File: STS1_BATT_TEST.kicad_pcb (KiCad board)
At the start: 2 copper layers, 81.8 x 46.9 mm, 6 parts, among them J1 TE 282834-6, J2 Conn_01x15

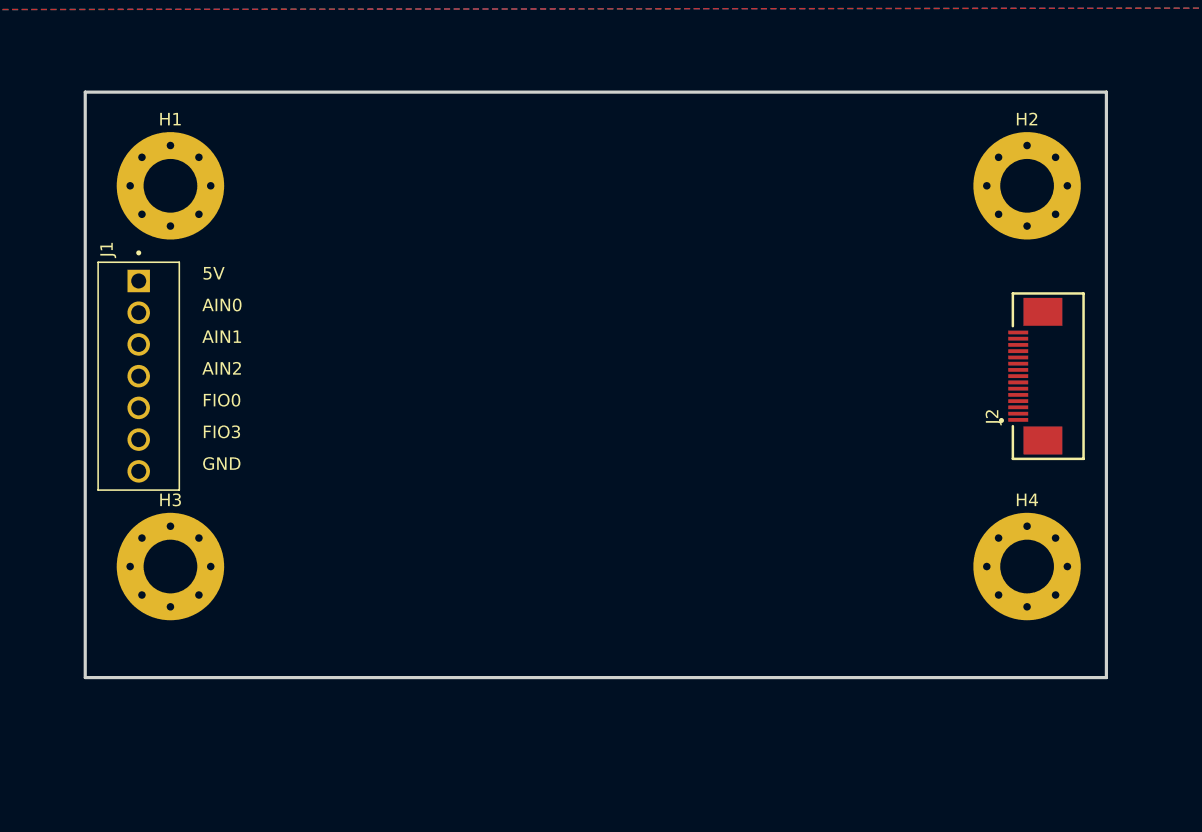
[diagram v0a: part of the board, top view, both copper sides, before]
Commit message: Prepared STS1_BATT_TEST.
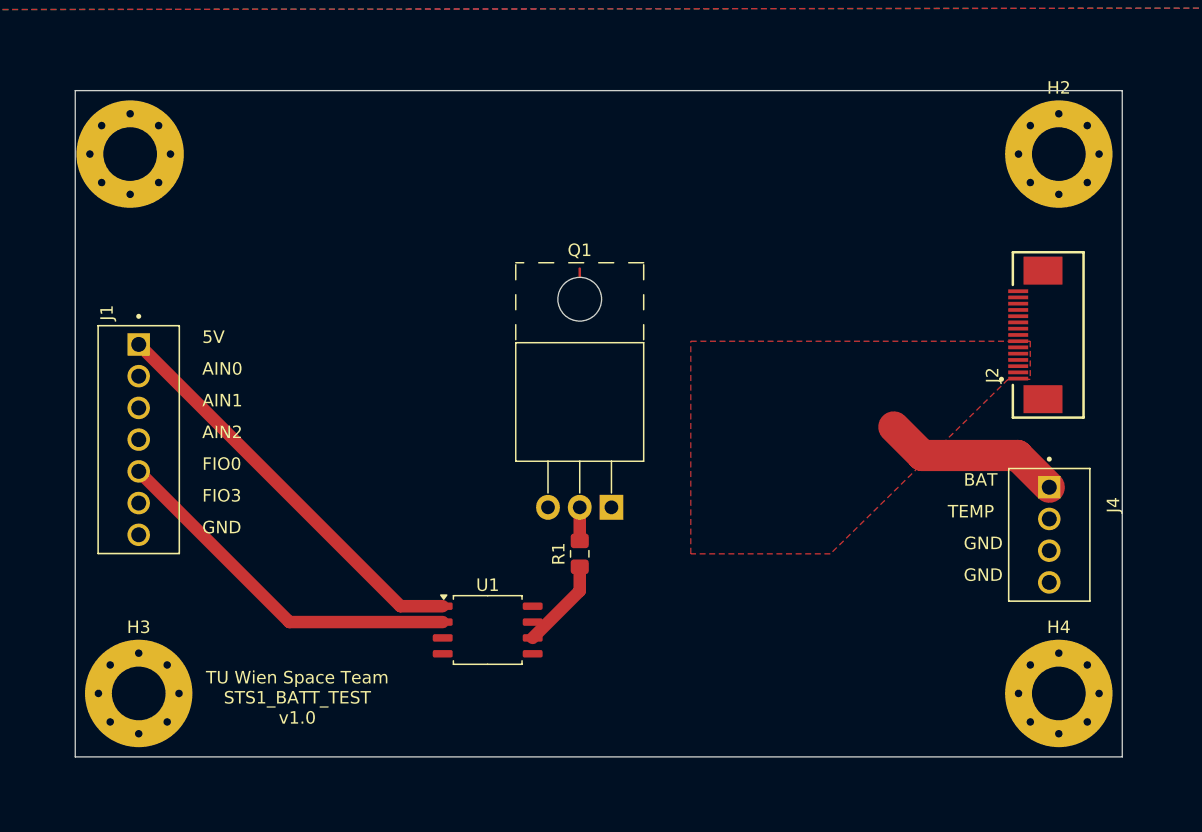
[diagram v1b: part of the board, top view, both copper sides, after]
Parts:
- added J4: Conn_01x04, STS1_Connectors:TE_282834-4, F.Cu at (154.2, 91.4)
- added Q1: IPP050N03LF2S, Package_TO_SOT_THT:TO-220-3_Horizontal_TabUp, F.Cu at (119.1, 89.2)
- added R1: 100, Capacitor_SMD:C_0805_2012Metric_Pad1.18x1.45mm_HandSolder, F.Cu at (116.6, 93.0)
- added U1: TC4420VOA713, Package_SO:SOIC-8_5.275x5.275mm_P1.27mm, F.Cu at (109.2, 99.1)
- moved H3 10.5 mm to (81.3, 104.1)
- moved H4 10.5 mm to (154.9, 104.1)
- moved J1 5.08 mm to (81.3, 83.8)
- moved H1 4.11 mm to (80.6, 61.0)
- moved H2 3.59 mm to (154.9, 61.0)
- moved J2 3.30 mm to (153.7, 75.4)
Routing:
- net +5V: track 0.00 -> 33.0 mm
- net /FIO0: track 0.00 -> 29.3 mm
- net /AIN0: track 0.00 -> 14.4 mm
- net /Load Mosfet with cooling/GATE: track 0.00 -> 7.25 mm
- net Net-(Q1-G): track 0.00 -> 5.56 mm
- added copper zone on F.Cu, net /AIN0
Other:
- board size 81.8 x 46.9 mm -> 83.8 x 53.3 mm
- board text added: "BAT"
- board text added: "TEMP"
- board text added: "TU Wien Space Team STS1_BATT_TEST v1.0"
